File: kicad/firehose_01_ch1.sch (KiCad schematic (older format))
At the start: 82 parts, among them J1 SMA, U1 MAX2112, U2 MAX19505, U20 MIC2090-1YM5, U3 MGA-68563

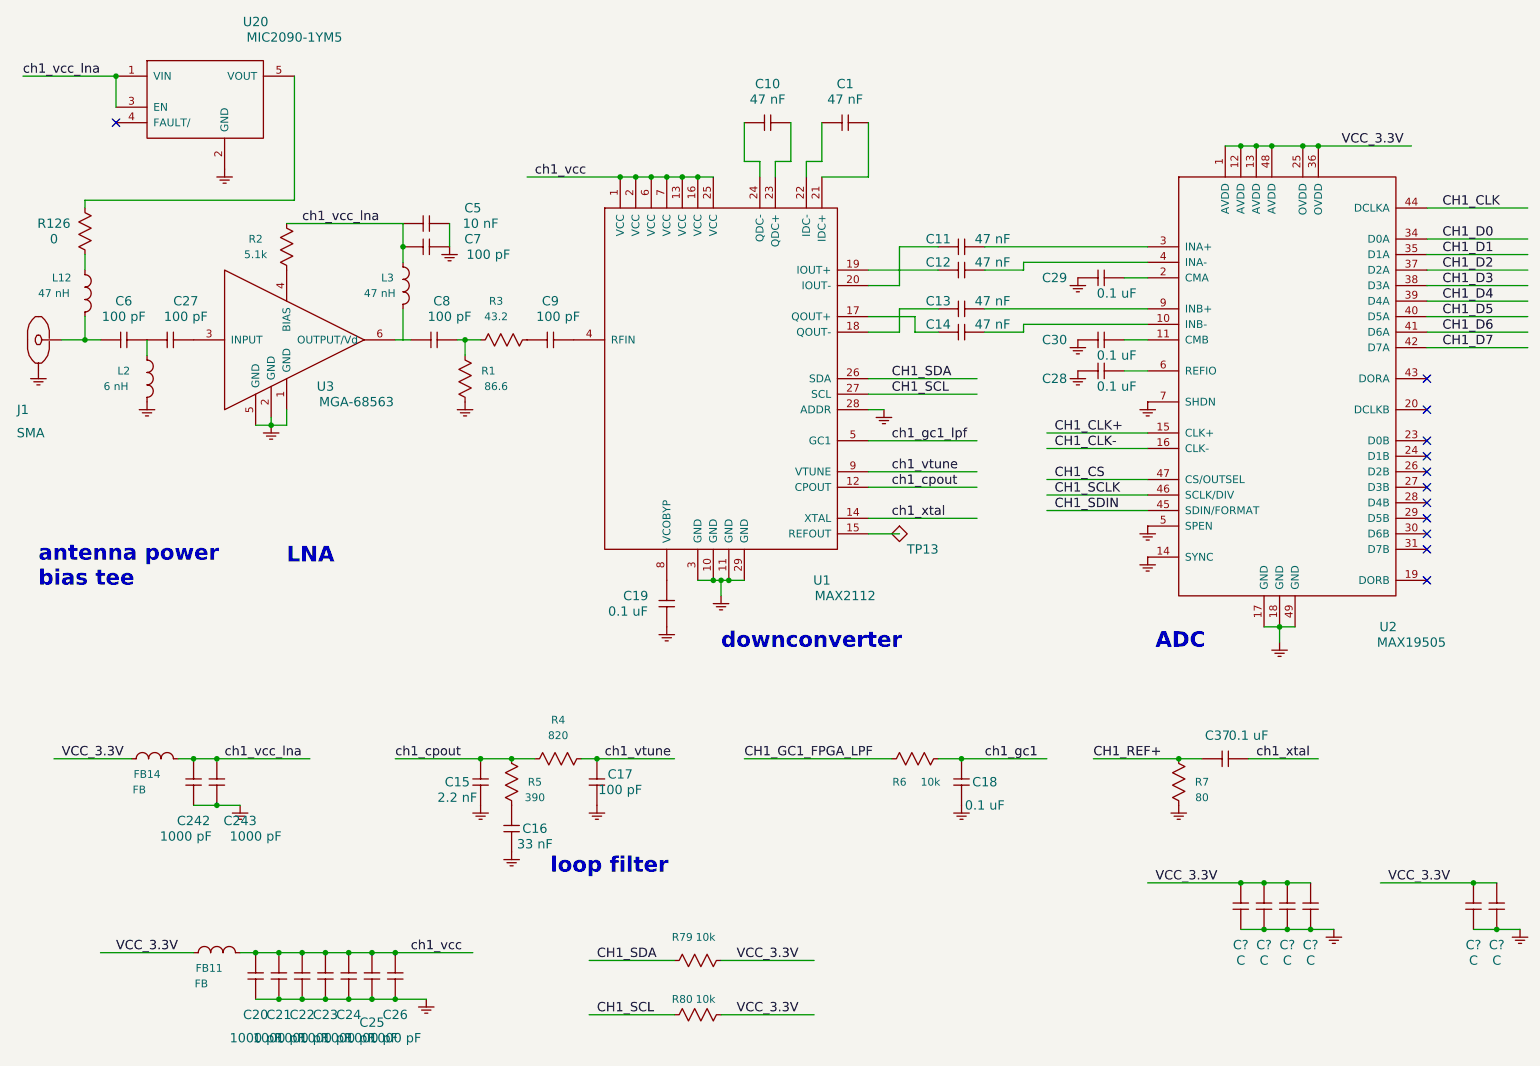
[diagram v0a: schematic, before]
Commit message: more KiCAD schematic
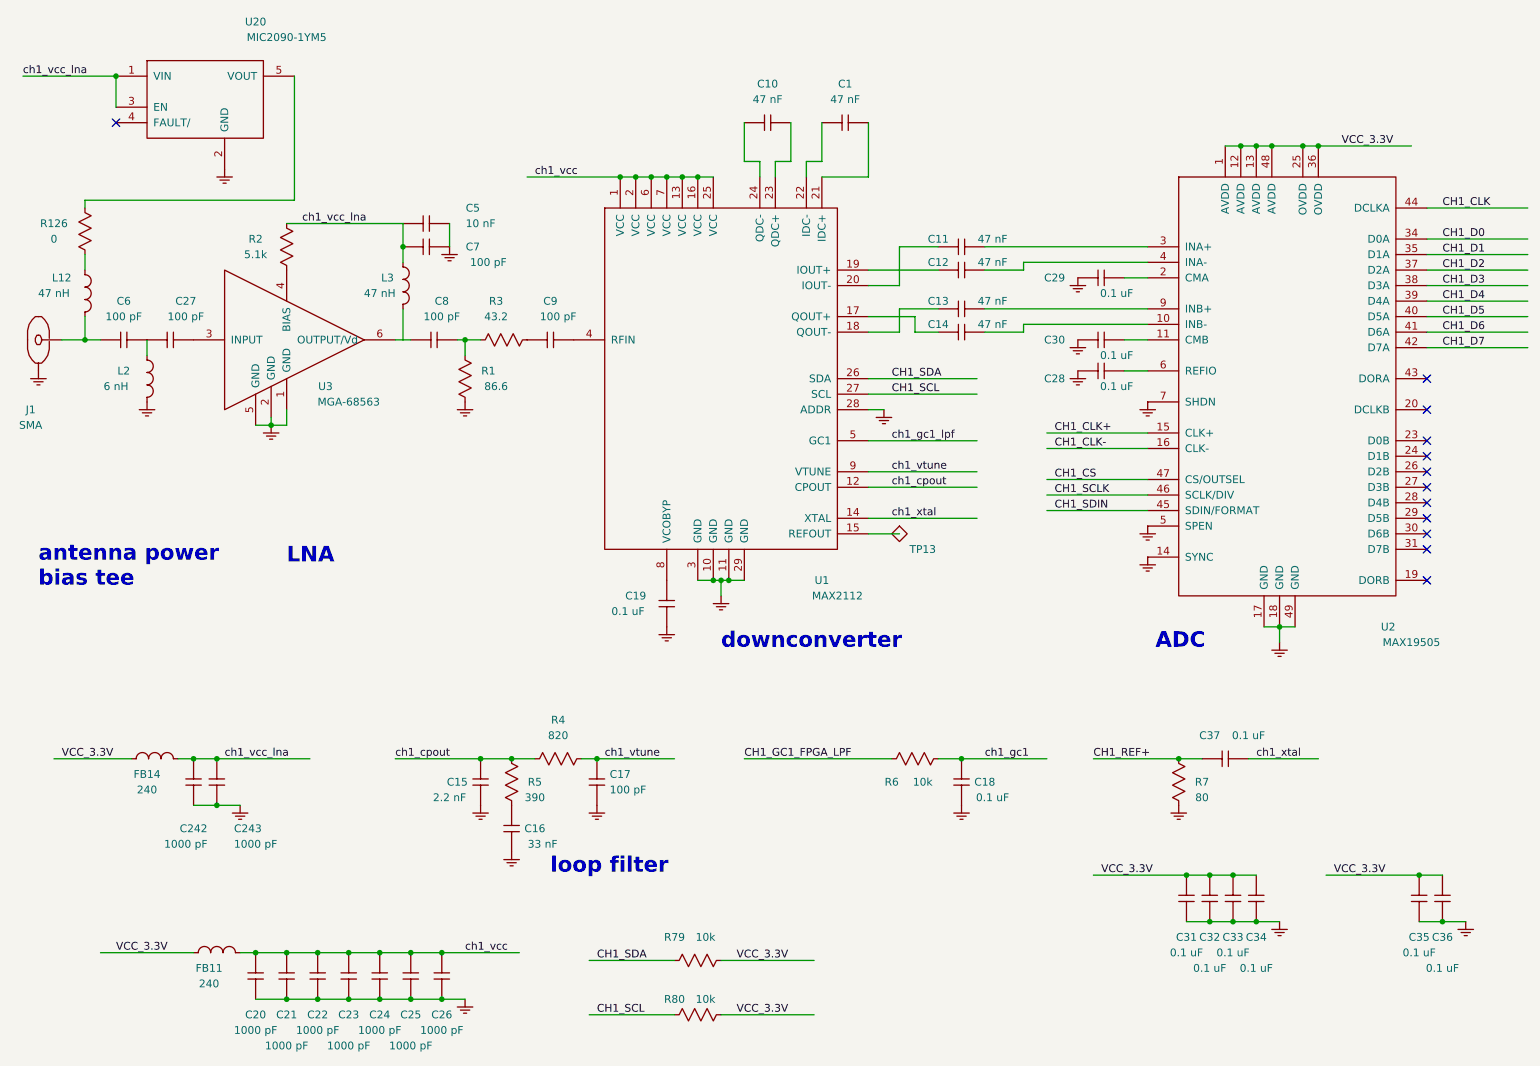
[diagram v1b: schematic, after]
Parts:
- C31, C32, C33, C34, C35, C36: renamed from C?; value C -> 0.1 uF
- FB11, FB14: value FB -> 240
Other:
- moved on the sheet: C21, C22, C23, C24, C25, C26, C31, C32, C33, C34, C35, C36
